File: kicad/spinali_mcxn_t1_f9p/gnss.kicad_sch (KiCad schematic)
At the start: 63 parts, among them J3 UART, SW1 SW_SPST, SW2 SW_SPST, U2 PCMF1USB3SZ, U3 AP2112K-3.3, U4 AP2112K-3.3, U5 NEO-F9P-15B

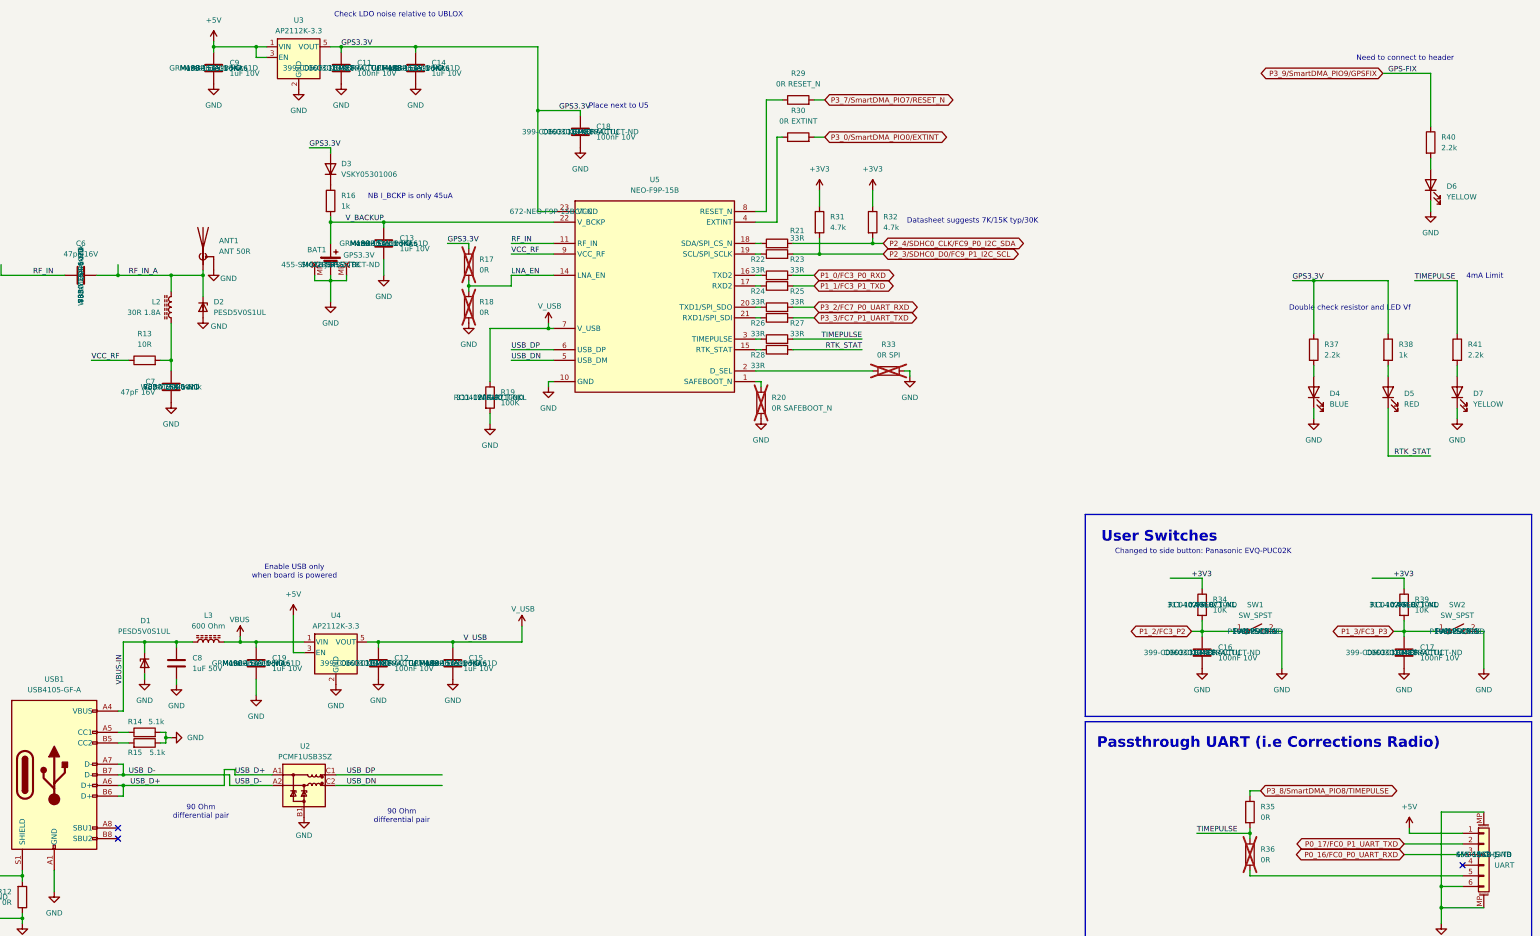
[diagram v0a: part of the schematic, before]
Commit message: Adjust pages and visibilty of part numbers
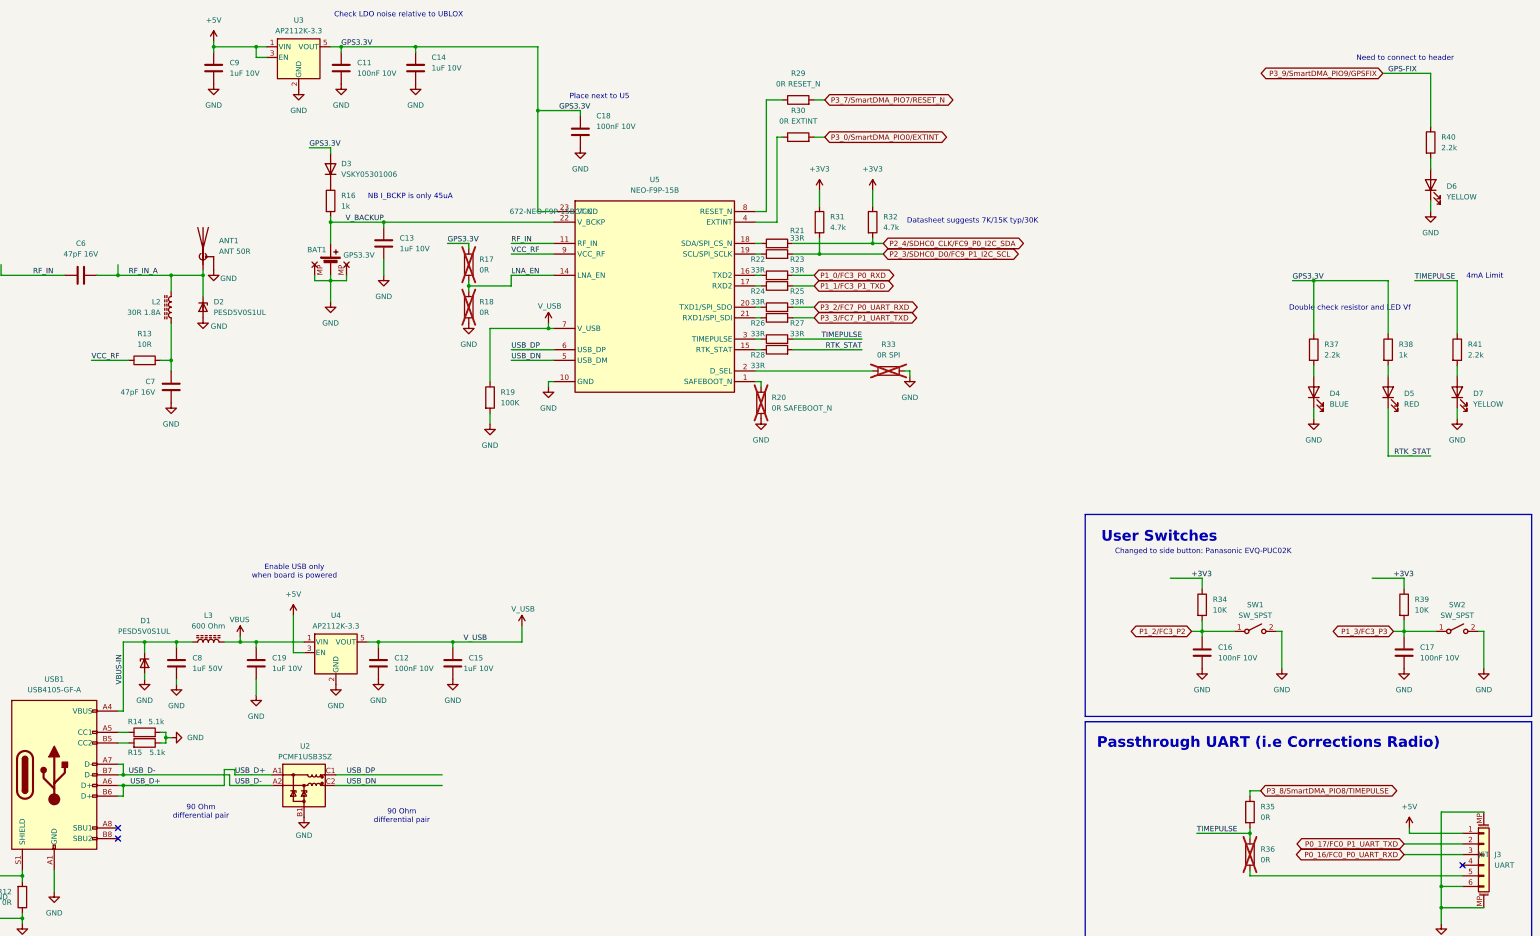
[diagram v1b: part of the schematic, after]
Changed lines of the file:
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@@
 	(text "Place next to U5"
 		(exclude_from_sim no)
-		(at 188.214 48.514 0)
+		(at 183.642 46.228 0)
 		(effects
 			(font
@@
 					(size 1.27 1.27)
 				)
+				(hide yes)
 			)
 		)
@@
 					(size 1.27 1.27)
 				)
+				(hide yes)
 			)
 		)
@@
 					(size 1.27 1.27)
 				)
+				(hide yes)
 			)
 		)
@@
 					(size 1.27 1.27)
 				)
+				(hide yes)
 			)
 		)
@@
 					(size 1.27 1.27)
 				)
+				(hide yes)
 			)
 		)
@@
 					(size 1.27 1.27)
 				)
+				(hide yes)
 			)
 		)
@@
 					(size 1.27 1.27)
 				)
+				(hide yes)
 			)
 		)
@@
 					(size 1.27 1.27)
 				)
+				(hide yes)
 			)
 		)
@@
 					(size 1.27 1.27)
 				)
+				(hide yes)
 			)
 		)
@@
 					(size 1.27 1.27)
 				)
+				(hide yes)
 			)
 		)
@@
 					(size 1.27 1.27)
 				)
+				(hide yes)
 			)
 		)
@@
 					(size 1.27 1.27)
 				)
+				(hide yes)
 			)
 		)
@@
 		(fields_autoplaced yes)
 		(property "Reference" "C18"
-			(at 182.88 53.3399 0)
+			(at 182.88 50.7999 0)
 			(effects
 				(font
@@
 		)
 		(property "Value" "100nF 10V"
-			(at 182.88 55.8799 0)
+			(at 182.88 53.3399 0)
 			(effects
 				(font
@@
 		)
 		(property "DigiKey" "399-C0603C104K8RACTUCT-ND"
-			(at 179.07 54.61 0)
+			(at 182.88 55.8799 0)
 			(effects
 				(font
 					(size 1.27 1.27)
 				)
+				(justify left)
+				(hide yes)
 			)
 		)
@@
 					(size 1.27 1.27)
 				)
+				(hide yes)
 			)
 		)
 		(property "MFPN" "C0603C104K8RACTU"
-			(at 179.07 54.61 0)
+			(at 182.88 58.4199 0)
 			(effects
 				(font
 					(size 1.27 1.27)
 				)
+				(justify left)
+				(hide yes)
 			)
 		)
@@
 					(size 1.27 1.27)
 				)
+				(hide yes)
 			)
 		)
@@
 					(size 1.27 1.27)
 				)
+				(hide yes)
 			)
 		)
@@
 					(size 1.27 1.27)
 				)
+				(hide yes)
 			)
 		)
@@
 					(size 1.27 1.27)
 				)
+				(hide yes)
 			)
 		)
@@
 					(size 1.27 1.27)
 				)
+				(hide yes)
 			)
 		)
@@
 					(size 1.27 1.27)
 				)
+				(hide yes)
 			)
 		)
@@
 					(size 1.27 1.27)
 				)
+				(hide yes)
 			)
 		)
@@
 					(size 1.27 1.27)
 				)
+				(hide yes)
 			)
 		)
@@
 					(size 1.27 1.27)
 				)
+				(hide yes)
 			)
 		)
@@
 					(size 1.27 1.27)
 				)
+				(hide yes)
 			)
 		)
@@
 					(size 1.27 1.27)
 				)
+				(hide yes)
 			)
 		)
@@
 		(fields_autoplaced yes)
 		(property "Reference" "C14"
-			(at 143.51 38.0999 0)
+			(at 143.51 36.8299 0)
 			(effects
 				(font
@@
 		)
 		(property "Value" "1uF 10V"
-			(at 143.51 40.6399 0)
+			(at 143.51 39.3699 0)
 			(effects
 				(font
@@
 					(size 1.27 1.27)
 				)
+				(hide yes)
 			)
 		)
 		(property "MF" "Murata Electronics"
-			(at 139.7 39.37 0)
+			(at 143.51 41.9099 0)
 			(effects
 				(font
 					(size 1.27 1.27)
 				)
+				(justify left)
+				(hide yes)
 			)
 		)
@@
 					(size 1.27 1.27)
 				)
+				(hide yes)
 			)
 		)
@@
 					(size 1.27 1.27)
 				)
+				(hide yes)
 			)
 		)
@@
 					(size 1.27 1.27)
 				)
+				(hide yes)
 			)
 		)
@@
 					(size 1.27 1.27)
 				)
+				(hide yes)
 			)
 		)
@@
 					(size 1.27 1.27)
 				)
+				(hide yes)
 			)
 		)
@@
 					(size 1.27 1.27)
 				)
+				(hide yes)
 			)
 		)
@@
 					(size 1.27 1.27)
 				)
+				(hide yes)
 			)
 		)
@@
 					(size 1.27 1.27)
 				)
+				(hide yes)
 			)
 		)
@@
 					(size 1.27 1.27)
 				)
+				(hide yes)
 			)
 		)
@@
 					(size 1.27 1.27)
 				)
+				(hide yes)
 			)
 		)
@@
 					(size 1.27 1.27)
 				)
+				(hide yes)
 			)
 		)
@@
 					(size 1.27 1.27)
 				)
+				(hide yes)
 			)
 		)
@@
 					(size 1.27 1.27)
 				)
+				(hide yes)
 			)
 		)
@@
 					(size 1.27 1.27)
 				)
+				(hide yes)
 			)
 		)
@@
 					(size 1.27 1.27)
 				)
+				(hide yes)
 			)
 		)
@@
 					(size 1.27 1.27)
 				)
+				(hide yes)
 			)
 		)
@@
 					(size 1.27 1.27)
 				)
+				(hide yes)
 			)
 		)
@@
 					(size 1.27 1.27)
 				)
+				(hide yes)
 			)
 		)
@@
 					(size 1.27 1.27)
 				)
+				(hide yes)
 			)
 		)
@@
 					(size 1.27 1.27)
 				)
+				(hide yes)
 			)
 		)
@@
 					(size 1.27 1.27)
 				)
+				(hide yes)
 			)
 		)
@@
 					(size 1.27 1.27)
 				)
+				(hide yes)
 			)
 		)
@@
 					(size 1.27 1.27)
 				)
+				(hide yes)
 			)
 		)
@@
 					(size 1.27 1.27)
 				)
+				(hide yes)
 			)
 		)
@@
 					(size 1.27 1.27)
 				)
+				(hide yes)
 			)
 		)
@@
 					(size 1.27 1.27)
 				)
+				(hide yes)
 			)
 		)
@@
 					(size 1.27 1.27)
 				)
+				(hide yes)
 			)
 		)
@@
 					(size 1.27 1.27)
 				)
+				(hide yes)
 			)
 		)
